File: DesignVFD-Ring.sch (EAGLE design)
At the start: 32 parts, among them IC1 LMR64010XMF/NOPB, IC2 LM340S-05, U1 MAX6920AWP+, U2 LM1084IS-5.0, U3 TPS76325DBVT

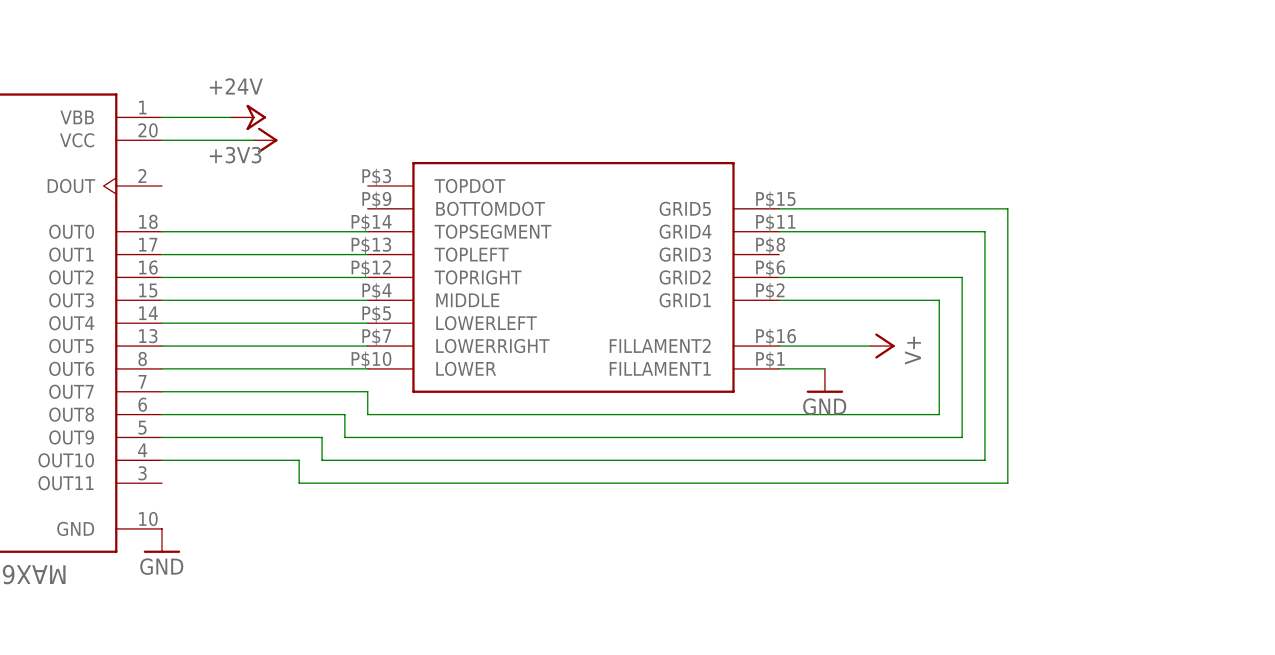
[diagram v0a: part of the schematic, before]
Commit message: IVL complete
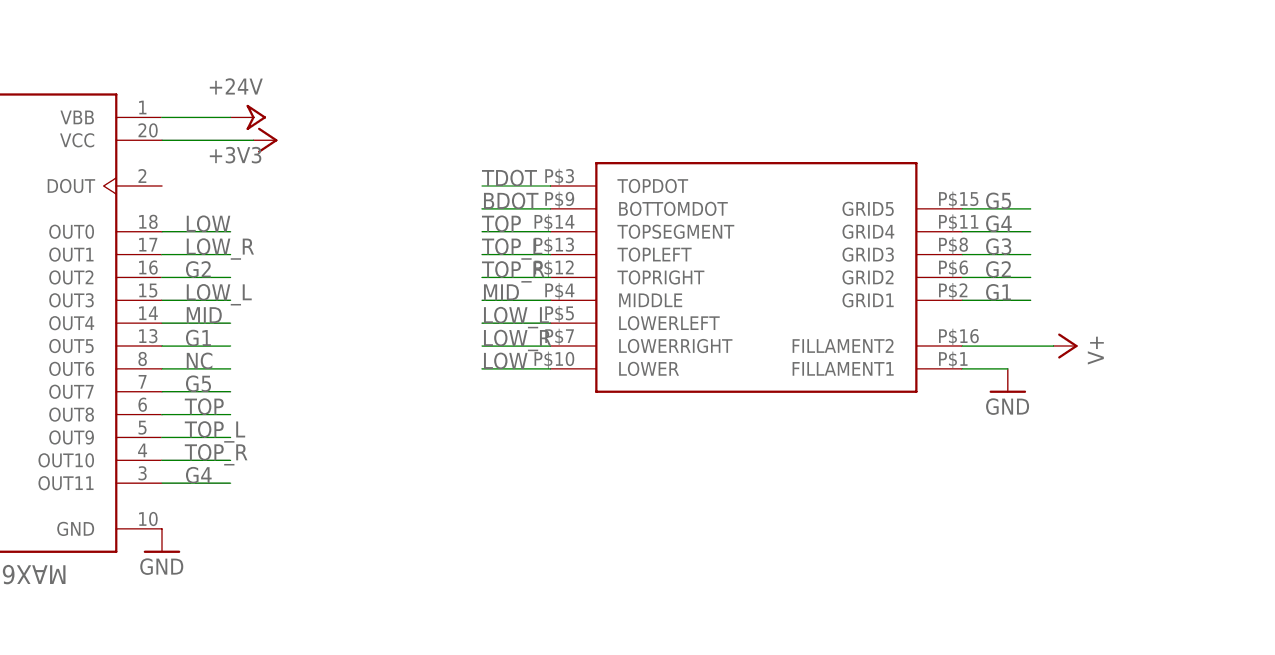
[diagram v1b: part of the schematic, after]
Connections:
- removed net N$10: U$2.MIDDLE, U1.OUT3
- removed net N$11: U$2.LOWERLEFT, U1.OUT4
- removed net N$12: U$2.LOWERRIGHT, U1.OUT5
- removed net N$13: U$2.LOWER, U1.OUT6
- removed net N$14: U$2.GRID1, U1.OUT7
- removed net N$15: U$2.GRID2, U1.OUT8
- removed net N$16: U$2.GRID4, U1.OUT9
- removed net N$17: U$2.GRID5, U1.OUT10
- removed net N$5: U$2.TOPSEGMENT, U1.OUT0
- removed net N$8: U$2.TOPLEFT, U1.OUT1
- removed net N$9: U$2.TOPRIGHT, U1.OUT2
- new net BDOT: U$2.BOTTOMDOT
- new net G1: U$2.GRID1, U1.OUT5
- new net G2: U$2.GRID2, U1.OUT2
- new net G3: U$2.GRID3
- new net G4: U$2.GRID4, U1.OUT11
- new net G5: U$2.GRID5, U1.OUT7
- new net LOW: U$2.LOWER, U1.OUT0
- new net LOW_L: U$2.LOWERLEFT, U1.OUT3
- new net LOW_R: U$2.LOWERRIGHT, U1.OUT1
- new net MID: U$2.MIDDLE, U1.OUT4
- new net NC: U1.OUT6
- new net TDOT: U$2.TOPDOT
- new net TOP: U$2.TOPSEGMENT, U1.OUT8
- new net TOP_L: U$2.TOPLEFT, U1.OUT9
- new net TOP_R: U$2.TOPRIGHT, U1.OUT10
